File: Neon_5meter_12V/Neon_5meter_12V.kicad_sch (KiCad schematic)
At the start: 7 parts, among them U1 ESP32-WROOM-32, U2 XL1509-3.3

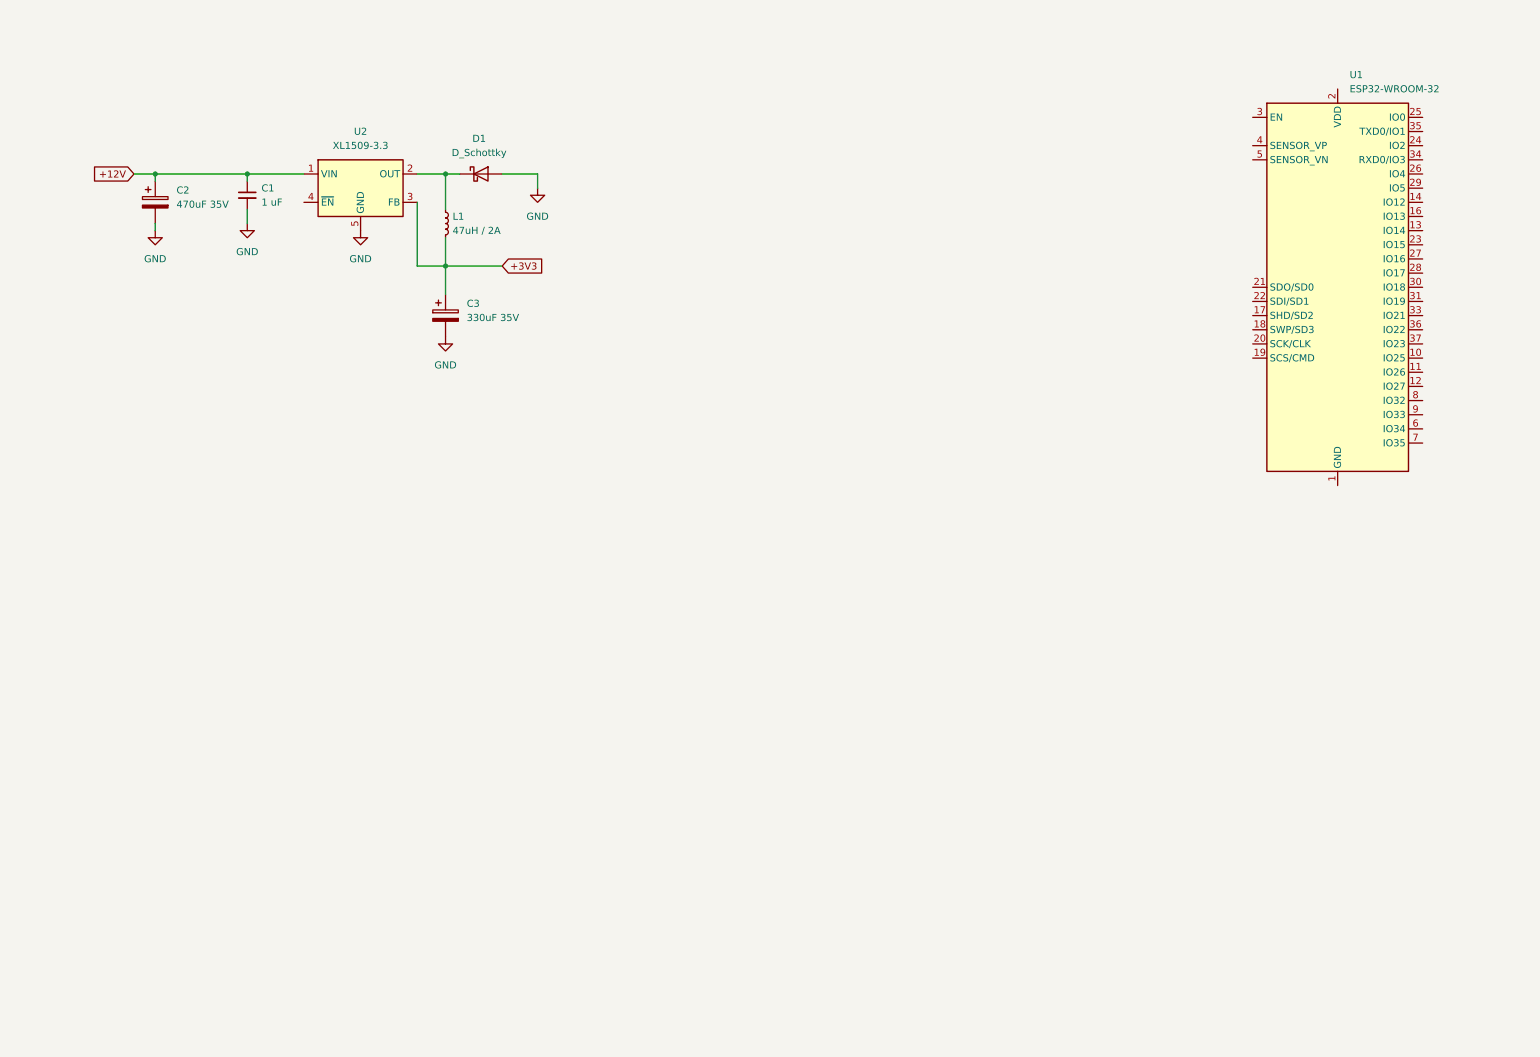
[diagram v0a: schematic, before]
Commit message: updated schematic
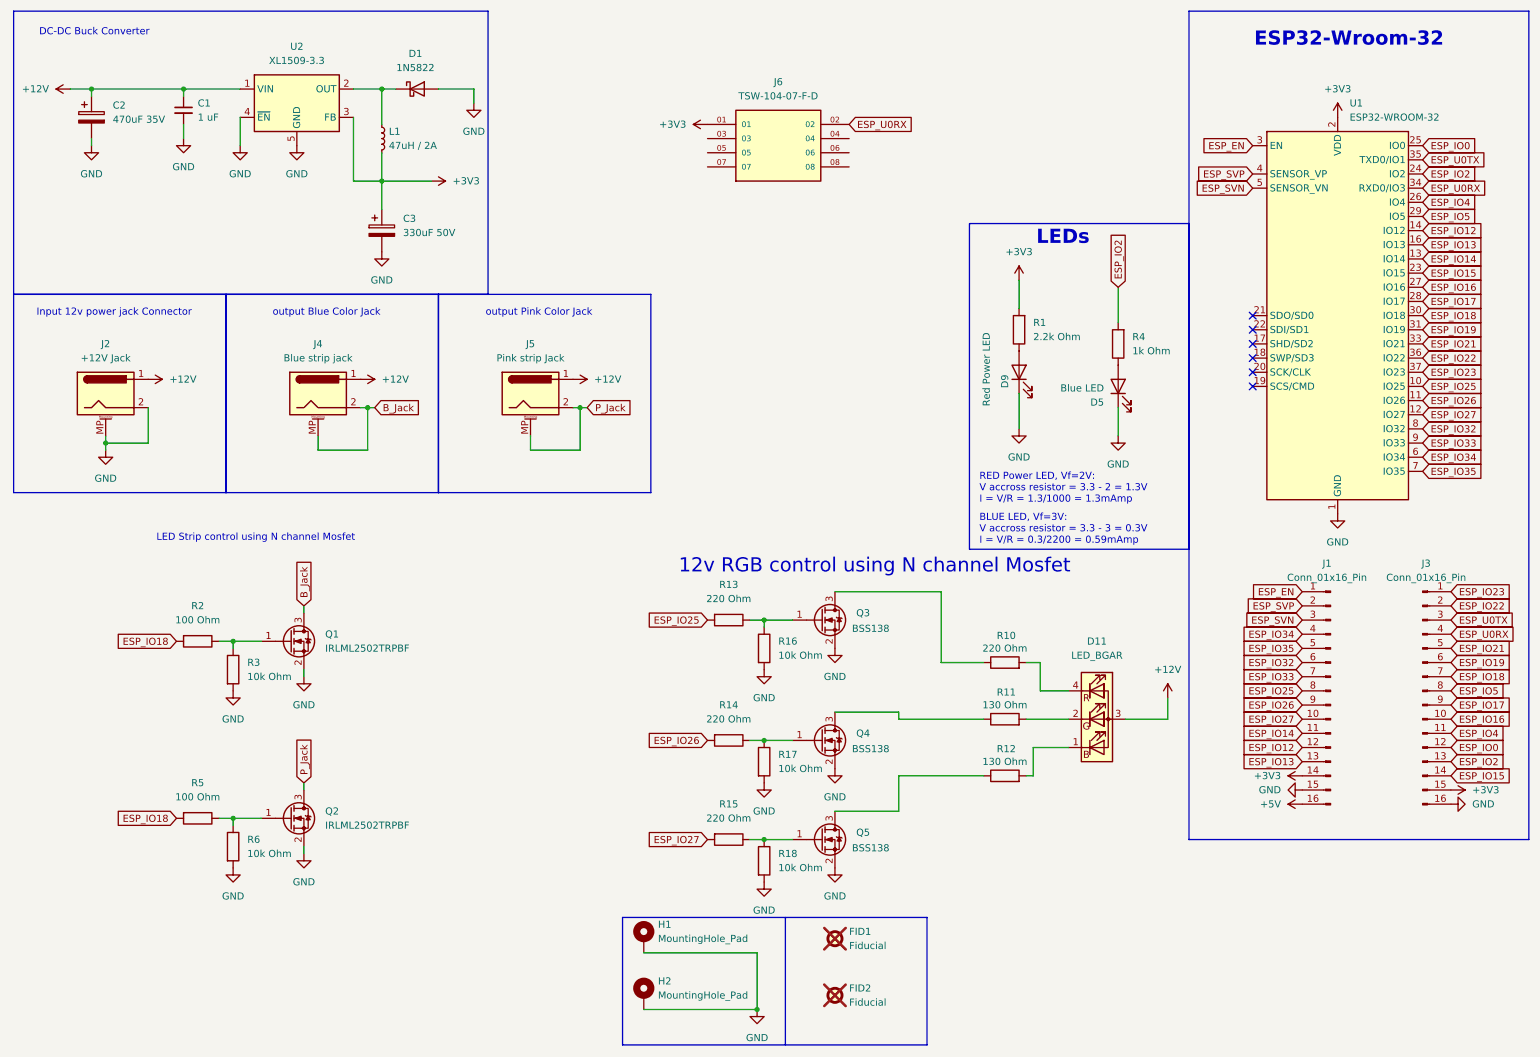
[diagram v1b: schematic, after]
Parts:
- added D11: LED_BGAR, LED_THT:LED_D5.0mm-4_RGB, symbol Device:LED_BGAR
- added D5: Blue LED, LED_SMD:LED_1206_3216Metric_Pad1.42x1.75mm_HandSolder, symbol Device:LED
- added D9: Red Power LED, LED_SMD:LED_1206_3216Metric_Pad1.42x1.75mm_HandSolder, symbol Device:LED
- added FID1, FID2: Fiducial, Fiducial:Fiducial_0.5mm_Mask1.5mm, symbol Mechanical:Fiducial
- added H1, H2: MountingHole_Pad, MountingHole:MountingHole_3.2mm_M3_Pad_Via, symbol Mechanical:MountingHole_Pad
- added J1, J3: Conn_01x16_Pin, Connector_PinHeader_2.54mm:PinHeader_1x16_P2.54mm_Vertical, symbol Connector:Conn_01x16_Pin
- added J2: +12V Jack, Connector_BarrelJack:BarrelJack_Horizontal, symbol Connector:Barrel_Jack_MountingPin
- added J4: Blue strip jack, Connector_BarrelJack:BarrelJack_Horizontal, symbol Connector:Barrel_Jack_MountingPin
- added J5: Pink strip Jack, Connector_BarrelJack:BarrelJack_Horizontal, symbol Connector:Barrel_Jack_MountingPin
- added J6: TSW-104-07-F-D, TSW-104-07-F-D:SAMTEC_TSW-104-07-F-D, symbol TSW-104-07-F-D:TSW-104-07-F-D
- added Q1, Q2: IRLML2502TRPBF, Package_TO_SOT_SMD:SOT-23, symbol Transistor_FET:BSS138
- added Q3, Q4, Q5: BSS138, Package_TO_SOT_SMD:SOT-23, symbol Transistor_FET:BSS138
- added R1: 2.2k Ohm, Resistor_SMD:R_1206_3216Metric_Pad1.30x1.75mm_HandSolder, symbol Device:R
- added R10, R13, R14, R15: 220 Ohm, Resistor_SMD:R_1206_3216Metric_Pad1.30x1.75mm_HandSolder, symbol Device:R
- added R11, R12: 130 Ohm, Resistor_SMD:R_1206_3216Metric_Pad1.30x1.75mm_HandSolder, symbol Device:R
- added R16, R17, R18, R3, R6: 10k Ohm, Resistor_SMD:R_1206_3216Metric_Pad1.30x1.75mm_HandSolder, symbol Device:R
- added R2, R5: 100 Ohm, Resistor_SMD:R_1206_3216Metric_Pad1.30x1.75mm_HandSolder, symbol Device:R
- added R4: 1k Ohm, Resistor_SMD:R_1206_3216Metric_Pad1.30x1.75mm_HandSolder, symbol Device:R
- C3: value 330uF 35V -> 330uF 50V
- D1: value D_Schottky -> 1N5822
- L1: value 47uH / 2A -> 47uH / 2A
- U1: link (none) -> https://uge-one.com/product/espressif-esp32-wroom-32-dual-c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
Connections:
- net +12V: now also D11.3 (A), J2.1, J4.1, J5.1
- net +3V3: now also U1.2 (VDD), J1.14 (Pin_14), J3.15 (Pin_15), J6.01, R1.2
- net GND: now also U1.1 (GND), U1.15 (GND), U1.38 (GND), U1.39 (GND), U2.4 (~{EN}), D5.1 (K), D9.1 (K), H1.1, H2.1, J1.15 (Pin_15), J2.2, J2.MP (MountPin), J3.16 (Pin_16), Q1.2 (S), Q2.2 (S), Q3.2 (S), Q4.2 (S), Q5.2 (S), R16.2, R17.2, R18.2, R3.2, R6.2
- net ESP_IO25: now reaches U1.10 (IO25)
- net ESP_IO25: now also J1.8 (Pin_8), R13.2
- net ESP_IO26: now reaches U1.11 (IO26)
- net ESP_IO26: now also J1.9 (Pin_9), R14.2
- net ESP_IO27: now reaches U1.12 (IO27)
- net ESP_IO27: now also J1.10 (Pin_10), R15.2
- net ESP_IO14: now reaches U1.13 (IO14)
- net ESP_IO14: now also J1.11 (Pin_11)
- net ESP_IO12: now reaches U1.14 (IO12)
- net ESP_IO12: now also J1.12 (Pin_12)
- net ESP_IO13: now reaches U1.16 (IO13)
- net ESP_IO13: now also J1.13 (Pin_13)
- net ESP_IO15: now reaches U1.23 (IO15)
- net ESP_IO15: now also J3.14 (Pin_14)
- net ESP_IO2: now reaches U1.24 (IO2)
- net ESP_IO2: now also J3.13 (Pin_13), R4.2
- net ESP_IO0: now reaches U1.25 (IO0)
- net ESP_IO0: now also J3.12 (Pin_12)
- net ESP_IO4: now reaches U1.26 (IO4)
- net ESP_IO4: now also J3.11 (Pin_11)
- net ESP_IO16: now reaches U1.27 (IO16)
- net ESP_IO16: now also J3.10 (Pin_10)
- net ESP_IO17: now reaches U1.28 (IO17)
- net ESP_IO17: now also J3.9 (Pin_9)
- net ESP_IO5: now reaches U1.29 (IO5)
- net ESP_IO5: now also J3.8 (Pin_8)
- net ESP_EN: now reaches U1.3 (EN)
- net ESP_EN: now also J1.1 (Pin_1)
- net ESP_IO18: now reaches U1.30 (IO18)
- net ESP_IO18: now also J3.7 (Pin_7), R2.2, R5.2
- net ESP_IO19: now reaches U1.31 (IO19)
- net ESP_IO19: now also J3.6 (Pin_6)
- net ESP_IO21: now reaches U1.33 (IO21)
- net ESP_IO21: now also J3.5 (Pin_5)
- net ESP_U0RX: now reaches U1.34 (RXD0/IO3)
- net ESP_U0RX: now also J3.4 (Pin_4), J6.02
- net ESP_U0TX: now reaches U1.35 (TXD0/IO1)
- net ESP_U0TX: now also J3.3 (Pin_3)
- net ESP_IO22: now reaches U1.36 (IO22)
- net ESP_IO22: now also J3.2 (Pin_2)
- net ESP_IO23: now reaches U1.37 (IO23)
- net ESP_IO23: now also J3.1 (Pin_1)
- net ESP_SVP: now reaches U1.4 (SENSOR_VP)
- net ESP_SVP: now also J1.2 (Pin_2)
- net ESP_SVN: now reaches U1.5 (SENSOR_VN)
- net ESP_SVN: now also J1.3 (Pin_3)
- net ESP_IO34: now reaches U1.6 (IO34)
- net ESP_IO34: now also J1.4 (Pin_4)
- net ESP_IO35: now reaches U1.7 (IO35)
- net ESP_IO35: now also J1.5 (Pin_5)
- net ESP_IO32: now reaches U1.8 (IO32)
- net ESP_IO32: now also J1.6 (Pin_6)
- net ESP_IO33: now reaches U1.9 (IO33)
- net ESP_IO33: now also J1.7 (Pin_7)
- new net: Q2.1 (G), R5.1, R6.1
- new net: Q3.1 (G), R13.1, R16.1
- new net: Q4.3 (D), R11.1
- new net: D11.2 (GK), R11.2
- new net: Q1.1 (G), R2.1, R3.1
- new net: Q5.3 (D), R12.1
- new net: D11.1 (BK), R12.2
- new net: Q5.1 (G), R15.1, R18.1
- new net: Q3.3 (D), R10.1
- new net: D11.4 (RK), R10.2
- new net: Q4.1 (G), R14.1, R17.1
- new net: D9.2 (A), R1.1
- new net: D5.2 (A), R4.1
- new net +5V: J1.16 (Pin_16)
- new net B_Jack: J4.2, J4.MP (MountPin), Q1.3 (D)
- new net P_Jack: J5.2, J5.MP (MountPin), Q2.3 (D)
- no-connect marks 0 -> 6
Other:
- note added: "12v RGB control using N channel Mosfet"
- note added: "BLUE LED, Vf=3V: V accross resistor = 3.3 - 3 = 0.3V I = V/R = 0.3/2200 = 0.59mAmp"
- note added: "DC-DC Buck Converter"
- note added: "ESP32-Wroom-32"
- note added: "Input 12v power jack Connector"
- note added: "LED Strip control using N channel Mosfet"
- note added: "LEDs"
- note added: "RED Power LED, Vf=2V: V accross resistor = 3.3 - 2 = 1.3V I = V/R = 1.3/1000 = 1.3mAmp"
- note added: "output Blue Color Jack"
- note added: "output Pink Color Jack"
- moved on the sheet: C1, C2, C3, D1, L1, U2
